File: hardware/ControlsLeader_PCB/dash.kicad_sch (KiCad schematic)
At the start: 6 parts

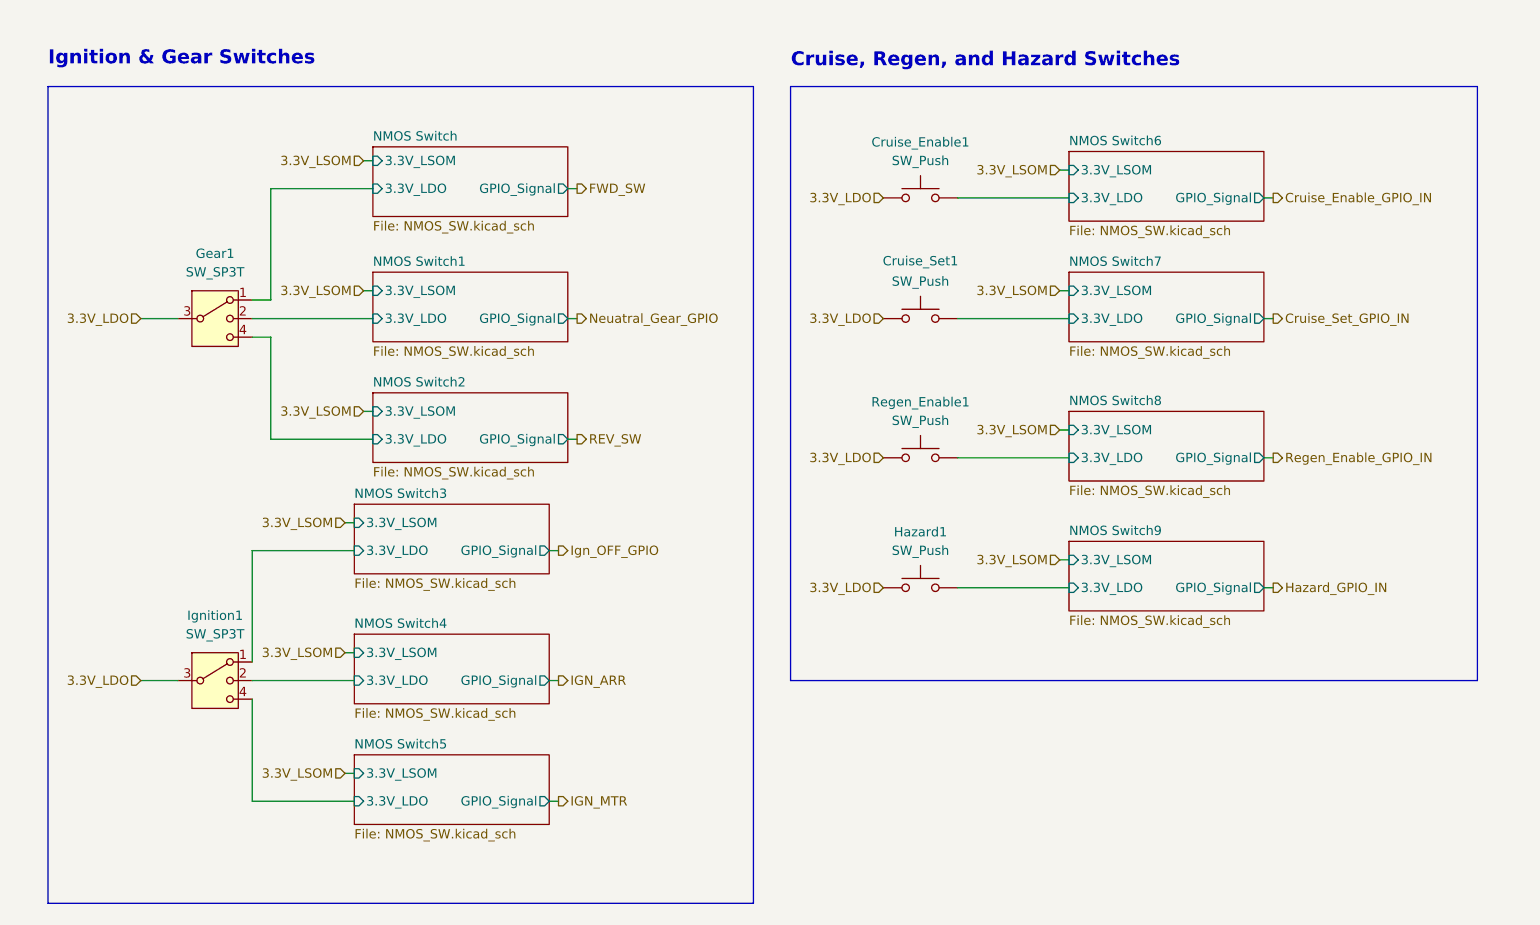
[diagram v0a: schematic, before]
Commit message: Ready for final review
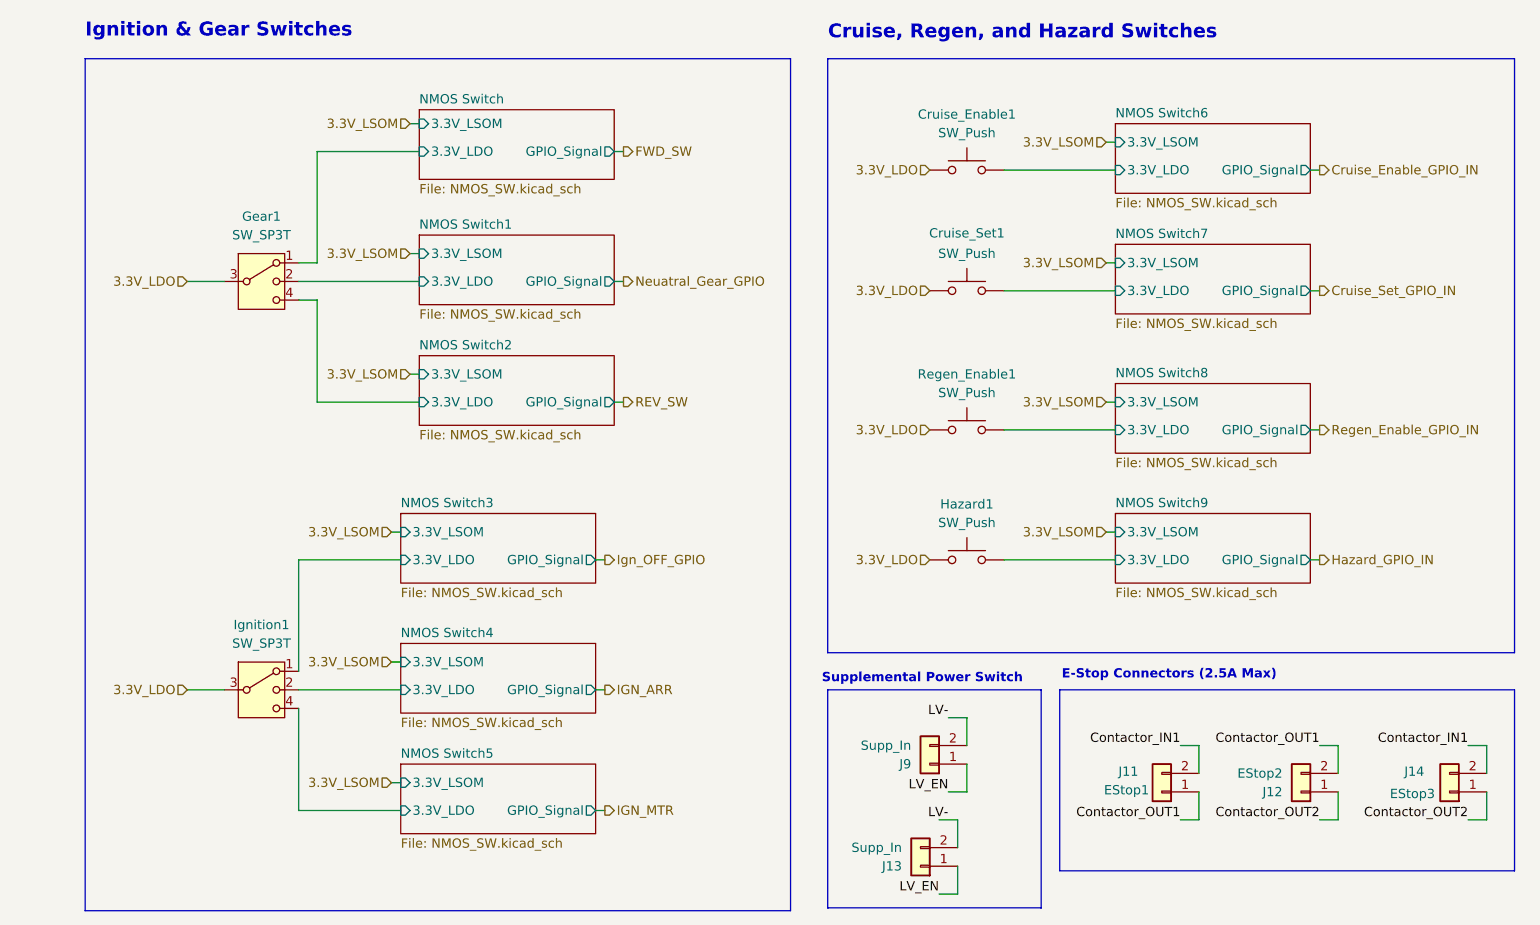
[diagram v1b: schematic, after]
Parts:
- added J11: EStop1, Connector_Molex:Molex_Micro-Fit_3.0_43650-0215_1x02_P3.00mm_Vertical, symbol Connector_Generic:Conn_01x02
- added J12: EStop2, Connector_Molex:Molex_Micro-Fit_3.0_43650-0215_1x02_P3.00mm_Vertical, symbol Connector_Generic:Conn_01x02
- added J13, J9: Supp_In, Connector_Molex:Molex_Micro-Fit_3.0_43650-0215_1x02_P3.00mm_Vertical, symbol Connector_Generic:Conn_01x02
- added J14: EStop3, Connector_Molex:Molex_Micro-Fit_3.0_43650-0215_1x02_P3.00mm_Vertical, symbol Connector_Generic:Conn_01x02
- Cruise_Enable1, Cruise_Set1, Hazard1, Regen_Enable1: Distributor Link (none) -> https://www.amazon.com/Gebildet-Waterproof-Momentary-Lockle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; Manufacturer (none) -> Amazon
- Gear1, Ignition1: Distributor Link (none) -> https://www.digikey.com/en/products/detail/c-k/A12505RNZQ/2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; Manufacturer (none) -> DigiKey
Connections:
- new net Contactor_IN1: J11.2 (Pin_2), J14.2 (Pin_2)
- new net Contactor_OUT1: J11.1 (Pin_1), J12.2 (Pin_2)
- new net Contactor_OUT2: J12.1 (Pin_1), J14.1 (Pin_1)
- new net LV-: J13.2 (Pin_2), J9.2 (Pin_2)
- new net LV_EN: J13.1 (Pin_1), J9.1 (Pin_1)
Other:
- note added: "E-Stop Connectors (2.5A Max)"
- note added: "Supplemental Power Switch"
- moved on the sheet: Cruise_Enable1, Cruise_Set1, Gear1, Hazard1, Ignition1, Regen_Enable1
